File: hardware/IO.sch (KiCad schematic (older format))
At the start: 15 parts, among them SW2 Interrupt, SW3 Port B, SW4 ~NMI

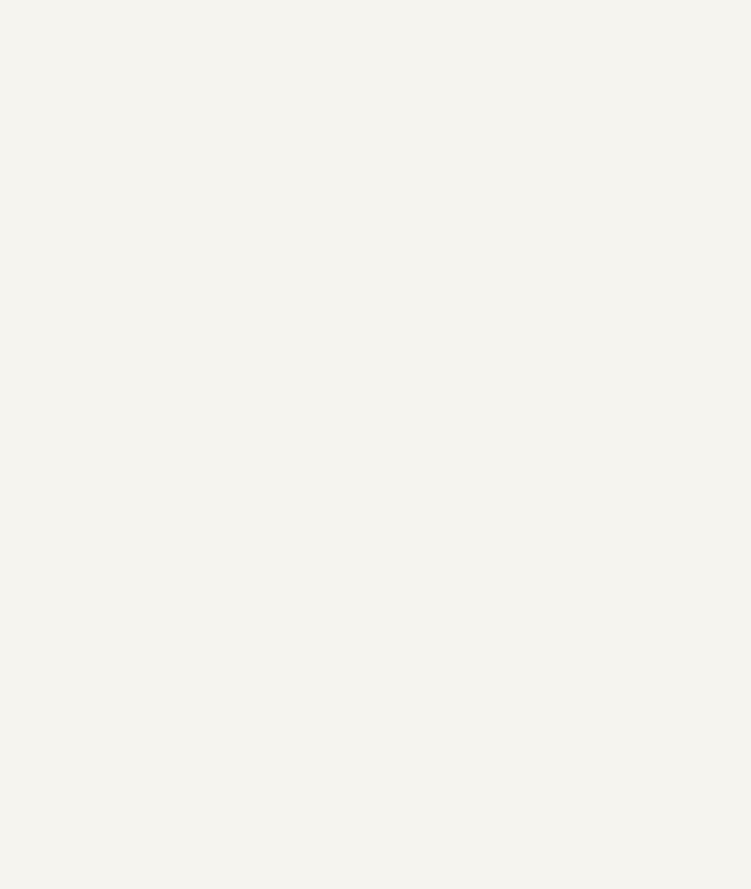
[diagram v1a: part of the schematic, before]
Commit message: Working on layout
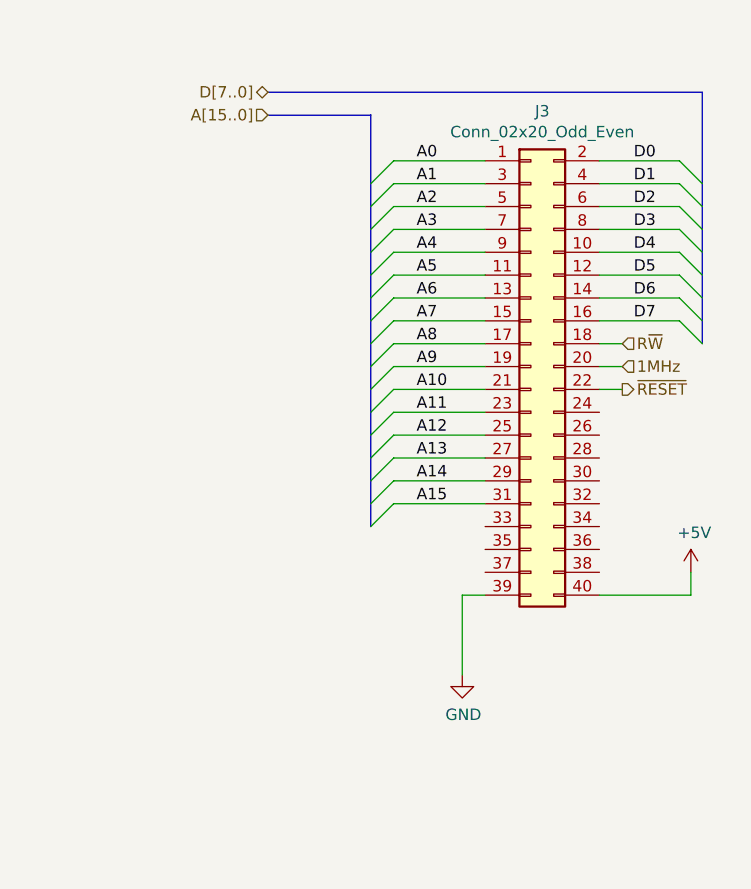
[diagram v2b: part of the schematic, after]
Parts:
- added J3: Conn_02x20_Odd_Even, Connector_PinHeader_2.54mm:PinHeader_2x20_P2.54mm_Horizontal, symbol Connector_Generic:Conn_02x20_Odd_Even
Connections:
- net +5V: now also J3.40 (Pin_40)
- net GND: now also J3.39 (Pin_39)
- new net 1MHz: J3.20 (Pin_20)
- new net A0: J3.1 (Pin_1)
- new net A1: J3.3 (Pin_3)
- new net A10: J3.21 (Pin_21)
- new net A11: J3.23 (Pin_23)
- new net A12: J3.25 (Pin_25)
- new net A13: J3.27 (Pin_27)
- new net A14: J3.29 (Pin_29)
- new net A15: J3.31 (Pin_31)
- new net A2: J3.5 (Pin_5)
- new net A3: J3.7 (Pin_7)
- new net A4: J3.9 (Pin_9)
- new net A5: J3.11 (Pin_11)
- new net A6: J3.13 (Pin_13)
- new net A7: J3.15 (Pin_15)
- new net A8: J3.17 (Pin_17)
- new net A9: J3.19 (Pin_19)
- new net D0: J3.2 (Pin_2)
- new net D1: J3.4 (Pin_4)
- new net D2: J3.6 (Pin_6)
- new net D3: J3.8 (Pin_8)
- new net D4: J3.10 (Pin_10)
- new net D5: J3.12 (Pin_12)
- new net D6: J3.14 (Pin_14)
- new net D7: J3.16 (Pin_16)
- new net R~W: J3.18 (Pin_18)
- new net ~RESET: J3.22 (Pin_22)
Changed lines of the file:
@@
 $Descr A4 11693 8268
 encoding utf-8
-Sheet 5 6
+Sheet 4 6
 Title "Retro PC"
 Date "2019-10-08"
@@
 Text HLabel 1600 6400 2    50   Output ~ 0
 ~NMI
+Text HLabel 10350 2150 2    50   Input ~ 0
+R~W
+Text HLabel 8800 1150 0    50   Input ~ 0
+A[15..0]
+Text HLabel 8800 1050 0    50   BiDi ~ 0
+D[7..0]
+Entry Wire Line
+	9250 1550 9350 1450
+Entry Wire Line
+	9250 1450 9350 1350
+Entry Wire Line
+	9250 1650 9350 1550
+Entry Wire Line
+	9250 1750 9350 1650
+Entry Wire Line
+	9250 1850 9350 1750
+Entry Wire Line
+	9250 1950 9350 1850
+Entry Wire Line
+	9250 2050 9350 1950
+Entry Wire Line
+	9250 2150 9350 2050
+Entry Wire Line
+	9250 2250 9350 2150
+Entry Wire Line
+	9250 2350 9350 2250
+Entry Wire Line
+	9350 2350 9250 2450
+Entry Wire Line
+	9250 2550 9350 2450
+Entry Wire Line
+	9250 2850 9350 2750
+Entry Wire Line
+	9350 2550 9250 2650
+Entry Wire Line
+	9250 2750 9350 2650
+Entry Wire Line
+	9250 2950 9350 2850
+Entry Wire Line
+	10700 1450 10600 1350
+Entry Wire Line
+	10700 1550 10600 1450
+Entry Wire Line
+	10700 1650 10600 1550
+Entry Wire Line
+	10700 1750 10600 1650
+Entry Wire Line
+	10700 1850 10600 1750
+Entry Wire Line
+	10700 1950 10600 1850
+Entry Wire Line
+	10700 2050 10600 1950
+Entry Wire Line
+	10700 2150 10600 2050
+Wire Wire Line
+	9350 1350 9750 1350
+Wire Wire Line
+	9350 1450 9750 1450
+Wire Wire Line
+	9350 1550 9750 1550
+Wire Wire Line
+	9350 1650 9750 1650
+Wire Wire Line
+	9350 1950 9750 1950
+Wire Wire Line
+	9350 2050 9750 2050
+Wire Wire Line
+	9350 2150 9750 2150
+Wire Wire Line
+	9350 2250 9750 2250
+Wire Wire Line
+	9350 2350 9750 2350
+Wire Wire Line
+	9350 2450 9750 2450
+Wire Wire Line
+	9350 2550 9750 2550
+Wire Wire Line
+	9350 2650 9750 2650
+Wire Wire Line
+	9350 2850 9750 2850
+Wire Wire Line
+	9350 2750 9750 2750
+Wire Wire Line
+	9350 1750 9750 1750
+Wire Wire Line
+	9350 1850 9750 1850
+Text Label 9450 1350 0    50   ~ 0
+A0
+Text Label 9450 1550 0    50   ~ 0
+A2
+Text Label 9450 1650 0    50   ~ 0
+A3
+Text Label 9450 1750 0    50   ~ 0
+A4
+Text Label 9450 1850 0    50   ~ 0
+A5
+Text Label 9450 1950 0    50   ~ 0
+A6
+Text Label 9450 2050 0    50   ~ 0
+A7
+Text Label 9450 2150 0    50   ~ 0
+A8
+Text Label 9450 2250 0    50   ~ 0
+A9
+Text Label 9450 2350 0    50   ~ 0
+A10
+Text Label 9450 2450 0    50   ~ 0
+A11
+Text Label 9450 2550 0    50   ~ 0
+A12
+Text Label 9450 2650 0    50   ~ 0
+A13
+Text Label 9450 2750 0    50   ~ 0
+A14
+Text Label 9450 2850 0    50   ~ 0
+A15
+Wire Wire Line
+	10250 1350 10600 1350
+Wire Wire Line
+	10250 1450 10600 1450
+Wire Wire Line
+	10250 1550 10600 1550
+Wire Wire Line
+	10250 1650 10600 1650
+Wire Wire Line
+	10250 1750 10600 1750
+Wire Wire Line
+	10250 1850 10600 1850
+Wire Wire Line
+	10250 1950 10600 1950
+Wire Wire Line
+	10250 2050 10600 2050
+Text Label 10400 1350 0    50   ~ 0
+D0
+Text Label 10400 1450 0    50   ~ 0
+D1
+Text Label 10400 1550 0    50   ~ 0
+D2
+Text Label 10400 1650 0    50   ~ 0
+D3
+Text Label 10400 1750 0    50   ~ 0
+D4
+Text Label 10400 1850 0    50   ~ 0
+D5
+Text Label 10400 1950 0    50   ~ 0
+D6
+Text Label 10400 2050 0    50   ~ 0
+D7
+$Comp
+L Connector_Generic:Conn_02x20_Odd_Even J3
+U 1 1 5DBDED7E
+P 9950 2250
+F 0 "J3" H 10000 3367 50  0000 C CNN
+F 1 "Conn_02x20_Odd_Even" H 10000 3276 50  0000 C CNN
+F 2 "Connector_PinHeader_2.54mm:PinHeader_2x20_P2.54mm_Horizontal" H 9950 2250 50  0001 C CNN
+F 3 "https://cdn.harwin.com/pdfs/M20-974.pdf" H 9950 2250 50  0001 C CNN
+F 4 "Harwin" H 9950 2250 50  0001 C CNN "Mfr."
+F 5 "M20-9742046" H 9950 2250 50  0001 C CNN "Mfr. No."
+F 6 "855-M20-9742046" H 9950 2250 50  0001 C CNN "Mouser"
+	1    9950 2250
+	1    0    0    -1
+$EndComp
+Wire Bus Line
+	9250 1150 8800 1150
+Wire Bus Line
+	8800 1050 10700 1050
+Wire Wire Line
+	10350 2150 10250 2150
+$Comp
+L power:GND #PWR?
+U 1 1 5DC0914B
+P 9650 3600
+AR Path="/5DC0914B" Ref="#PWR?"  Part="1"
+AR Path="/5EB09E21/5DC0914B" Ref="#PWR?"  Part="1"
+AR Path="/5EC67F7B/5DC0914B" Ref="#PWR070"  Part="1"
+F 0 "#PWR070" H 9650 3350 50  0001 C CNN
+F 1 "GND" H 9655 3427 50  0000 C CNN
+F 2 "" H 9650 3600 50  0001 C CNN
+F 3 "" H 9650 3600 50  0001 C CNN
+	1    9650 3600
+	1    0    0    -1
+$EndComp
+Wire Wire Line
+	9650 3600 9650 3250
+Wire Wire Line
+	9750 3250 9650 3250
+$Comp
+L power:+5V #PWR?
+U 1 1 5DC11208
+P 10650 3150
+AR Path="/5DC11208" Ref="#PWR?"  Part="1"
+AR Path="/5EB09E21/5DC11208" Ref="#PWR?"  Part="1"
+AR Path="/5EC67F7B/5DC11208" Ref="#PWR071"  Part="1"
+F 0 "#PWR071" H 10650 3000 50  0001 C CNN
+F 1 "+5V" H 10665 3323 50  0000 C CNN
+F 2 "" H 10650 3150 50  0001 C CNN
+F 3 "" H 10650 3150 50  0001 C CNN
+	1    10650 3150
+	1    0    0    -1
+$EndComp
+Wire Wire Line
+	10650 3150 10650 3250
+Wire Wire Line
+	10250 3250 10650 3250
+Text Label 9450 1450 0    50   ~ 0
+A1
+Text HLabel 10350 2250 2    50   Input ~ 0
+1MHz
+Wire Wire Line
+	10350 2250 10250 2250
+Text HLabel 10350 2350 2    50   Output ~ 0
+~RESET
+Wire Wire Line
+	10350 2350 10250 2350
 Wire Bus Line
 	2850 3450 2850 4150
 Wire Bus Line
 	1800 1000 1800 1700
+Wire Bus Line
+	10700 1050 10700 2150
+Wire Bus Line
+	9250 1150 9250 2950
 $EndSCHEMATC
